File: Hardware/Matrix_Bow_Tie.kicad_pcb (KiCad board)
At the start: 2 copper layers, 17.8 x 13 mm, 9 parts, among them U1 MAX4466

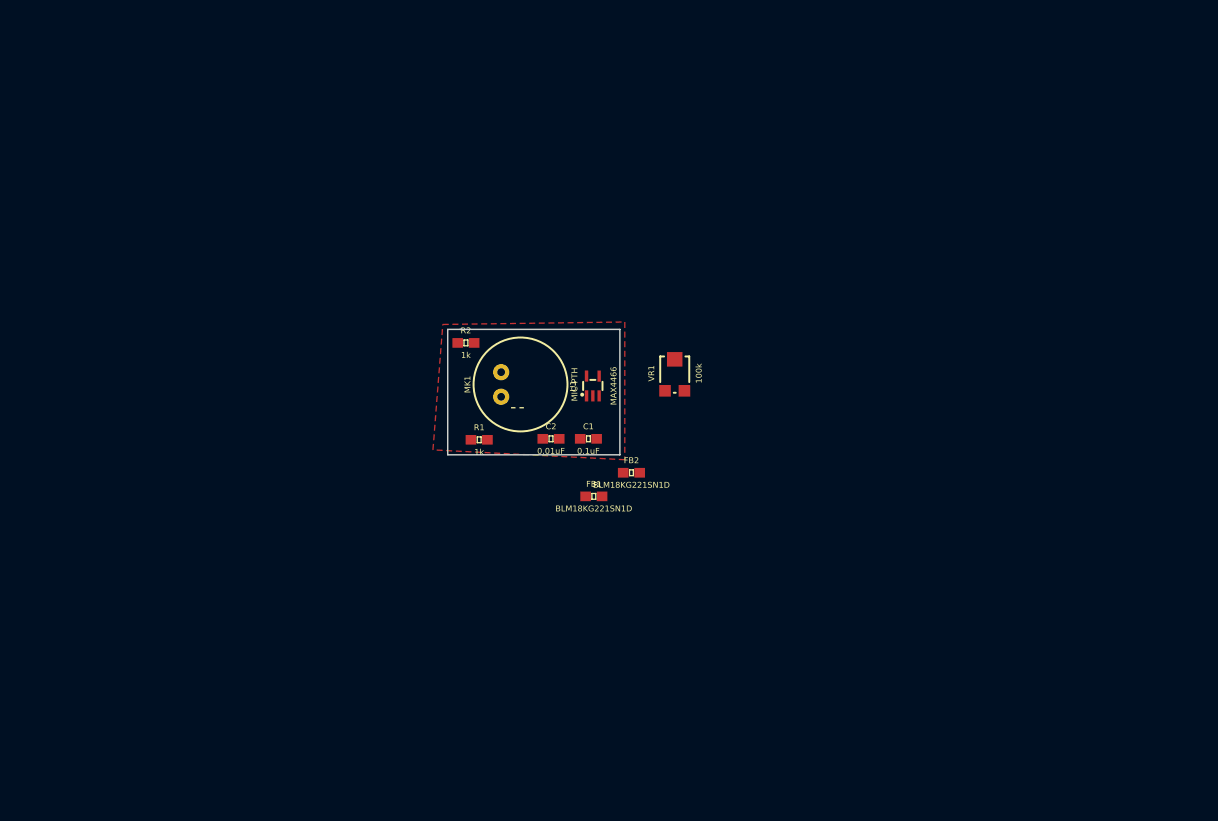
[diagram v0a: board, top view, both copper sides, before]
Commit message: Parts mostly laid out
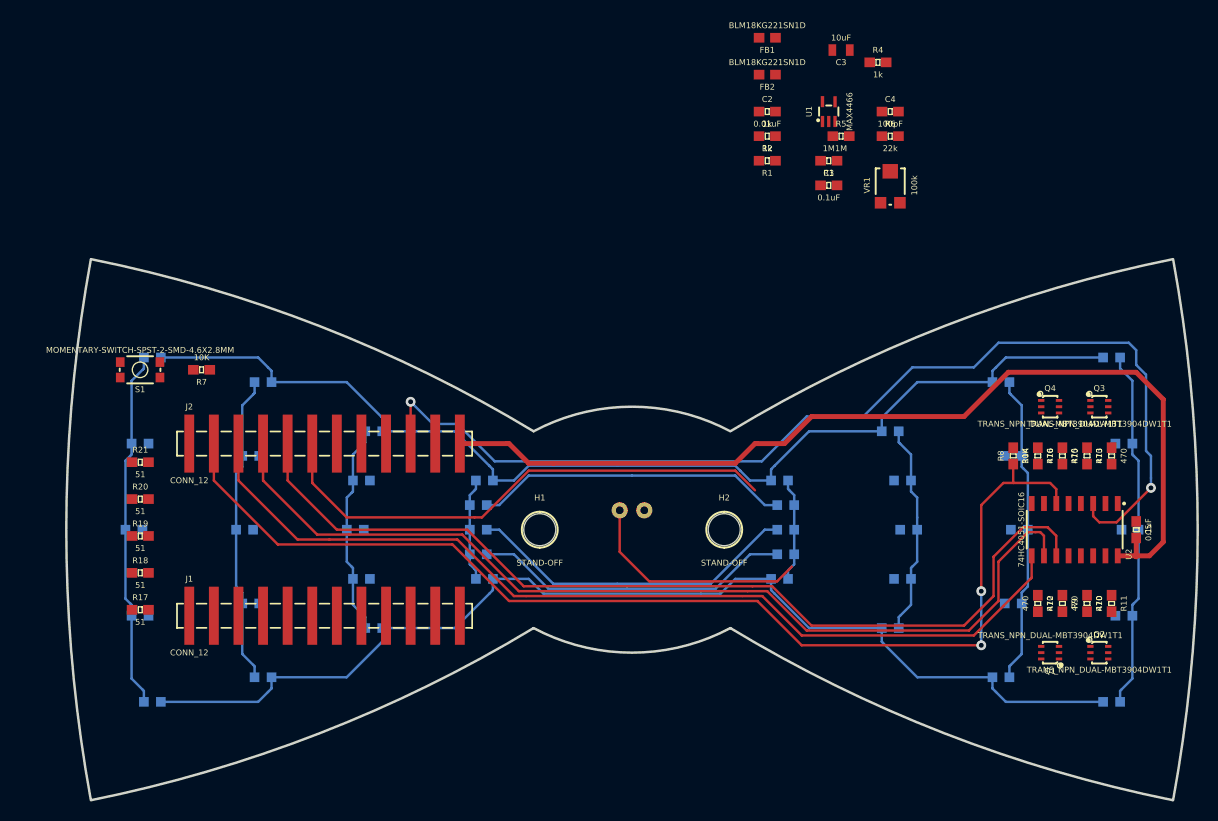
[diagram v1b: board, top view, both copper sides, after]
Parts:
- added C3: 10uF, Capacitors:0805, F.Cu at (181.6, 70.5)
- added C4: 100pF, Capacitors:0603, F.Cu at (186.7, 76.8)
- added C5: 0.1uF, Capacitors:0603, F.Cu at (212.1, 120.0)
- added D1: Yellow, LED:LED-0603, B.Cu at (209.5, 102.2)
- added D10: Yellow, LED:LED-0603, B.Cu at (198.1, 135.2)
- added D11: Yellow, LED:LED-0603, B.Cu at (186.7, 109.8)
- added D12: Yellow, LED:LED-0603, B.Cu at (187.9, 114.9)
- added D13: Yellow, LED:LED-0603, B.Cu at (188.6, 120.0)
- added D14: Yellow, LED:LED-0603, B.Cu at (187.9, 125.1)
- added D15: Yellow, LED:LED-0603, B.Cu at (186.7, 130.2)
- added D16: Yellow, LED:LED-0603, B.Cu at (175.2, 114.9)
- added D17: Yellow, LED:LED-0603, B.Cu at (175.9, 117.5)
- added D18: Yellow, LED:LED-0603, B.Cu at (175.9, 120.0)
- added D19: Yellow, LED:LED-0603, B.Cu at (175.9, 122.5)
- added D2: Yellow, LED:LED-0603, B.Cu at (210.8, 111.1)
- added D20: Yellow, LED:LED-0603, B.Cu at (175.2, 125.1)
- added D21: Yellow, LED:LED-0603, B.Cu at (144.8, 114.9)
- added D22: Yellow, LED:LED-0603, B.Cu at (144.1, 117.5)
- added D23: Yellow, LED:LED-0603, B.Cu at (144.1, 120.0)
- added D24: Yellow, LED:LED-0603, B.Cu at (144.1, 122.5)
- added D25: Yellow, LED:LED-0603, B.Cu at (144.8, 125.1)
- added D26: Yellow, LED:LED-0603, B.Cu at (133.3, 109.8)
- added D27: Yellow, LED:LED-0603, B.Cu at (132.1, 114.9)
- added D28: Yellow, LED:LED-0603, B.Cu at (131.4, 120.0)
- added D29: Yellow, LED:LED-0603, B.Cu at (132.1, 125.1)
- added D3: Yellow, LED:LED-0603, B.Cu at (211.4, 120.0)
- added D30: Yellow, LED:LED-0603, B.Cu at (133.3, 130.2)
- added D31: Yellow, LED:LED-0603, B.Cu at (121.9, 104.8)
- added D32: Yellow, LED:LED-0603, B.Cu at (120.6, 112.4)
- added D33: Yellow, LED:LED-0603, B.Cu at (120.0, 120.0)
- added D34: Yellow, LED:LED-0603, B.Cu at (120.6, 127.6)
- added D35: Yellow, LED:LED-0603, B.Cu at (121.9, 135.2)
- added D36: Yellow, LED:LED-0603, B.Cu at (110.5, 102.2)
- added D37: Yellow, LED:LED-0603, B.Cu at (109.2, 111.1)
- added D38: Yellow, LED:LED-0603, B.Cu at (108.6, 120.0)
- added D39: Yellow, LED:LED-0603, B.Cu at (109.2, 128.9)
- added D4: Yellow, LED:LED-0603, B.Cu at (210.8, 128.9)
- added D40: Yellow, LED:LED-0603, B.Cu at (110.5, 137.8)
- added D5: Yellow, LED:LED-0603, B.Cu at (209.5, 137.8)
- added D6: Yellow, LED:LED-0603, B.Cu at (198.1, 104.8)
- added D7: Yellow, LED:LED-0603, B.Cu at (199.4, 112.4)
- added D8: Yellow, LED:LED-0603, B.Cu at (200.0, 120.0)
- added D9: Yellow, LED:LED-0603, B.Cu at (199.4, 127.6)
- added H1: STAND-OFF, STAND-OFF, F.Cu at (150.5, 120.0)
- added H2: STAND-OFF, STAND-OFF, F.Cu at (169.5, 120.0)
- added J1: CONN_12, Matrix_Bot_Tie:1X12_SMD_MALE, F.Cu at (114.3, 128.9)
- added J2: CONN_12, Matrix_Bot_Tie:1X12_SMD_MALE, F.Cu at (114.3, 111.1)
- added Q1: TRANS_NPN_DUAL-MBT3904DW1T1, Silicon-Standard:SC70-6, F.Cu at (203.2, 132.7)
- added Q2: TRANS_NPN_DUAL-MBT3904DW1T1, Silicon-Standard:SC70-6, F.Cu at (208.3, 132.7)
- added Q3: TRANS_NPN_DUAL-MBT3904DW1T1, Silicon-Standard:SC70-6, F.Cu at (208.3, 107.3)
- added Q4: TRANS_NPN_DUAL-MBT3904DW1T1, Silicon-Standard:SC70-6, F.Cu at (203.2, 107.3)
- added R10: 470, Resistors:0603, F.Cu at (207.0, 127.6)
- added R11: 470, Resistors:0603, F.Cu at (209.5, 127.6)
- added R12: 470, Resistors:0603, F.Cu at (201.9, 127.6)
- added R13: 470, Resistors:0603, F.Cu at (209.5, 112.4)
- added R14: 470, Resistors:0603, F.Cu at (201.9, 112.4)
- added R15: 470, Resistors:0603, F.Cu at (207.0, 112.4)
- added R16: 470, Resistors:0603, F.Cu at (204.4, 112.4)
- added R17: 51, Resistors:0603, F.Cu at (109.2, 128.3)
- added R18: 51, Resistors:0603, F.Cu at (109.2, 124.5)
- added R19: 51, Resistors:0603, F.Cu at (109.2, 120.7)
- added R20: 51, Resistors:0603, F.Cu at (109.2, 116.8)
- added R21: 51, Resistors:0603, F.Cu at (109.2, 113.0)
- added R3: 1M, Resistors:0603, F.Cu at (180.3, 81.9)
- added R4: 1k, Resistors:0603, F.Cu at (185.4, 71.7)
- added R5: 1M, Resistors:0603, F.Cu at (181.6, 79.4)
- added R6: 22k, Resistors:0603, F.Cu at (186.7, 79.4)
- added R7: 10K, Resistors:0603, F.Cu at (115.5, 103.5)
- added R8: 10K, Resistors:0603, F.Cu at (199.4, 112.4)
- added R9: 470, Resistors:0603, F.Cu at (204.4, 127.6)
- added S1: MOMENTARY-SWITCH-SPST-2-SMD-4.6X2.8MM, Switches:TACTILE_SWITCH_SMD_4.6X2.8MM, F.Cu at (109.2, 103.5)
- added U2: 74HC4051-SOIC16, Matrix_Bot_Tie:SOIC-16, F.Cu at (205.7, 120.0)
- C1, C2: footprint 0603 -> Capacitors:0603
- FB1, FB2: footprint 0603 -> Coils:0603
- MK1: footprint MICROPHONE-PTH-9.7MM -> Silicon-Custom:MICROPHONE-PTH-9.7MM; moved to B.Cu
- R1, R2: footprint 0603 -> Resistors:0603
- VR1: footprint TC33X -> Matrix_Bot_Tie:TC33X
- moved FB1 50.6 mm to (174.0, 69.2), turned to 180 degrees
- moved FB2 43.4 mm to (174.0, 73.0), turned to 180 degrees
- moved R1 41.4 mm to (174.0, 81.9), turned to 180 degrees
- moved C2 40.5 mm to (174.0, 76.8)
- moved R2 37.7 mm to (174.0, 79.4), turned to 180 degrees
- moved U1 37.4 mm to (180.3, 76.8)
- moved C1 36.1 mm to (180.3, 84.4)
- moved VR1 29.5 mm to (186.7, 84.4)
- moved MK1 18.9 mm to (160.0, 120.0), turned to 270 degrees
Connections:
- U1 pad 1: Net-(U1-Pad1) -> Net-(C2-Pad2)
- U1 pad 4: Net-(U1-Pad4) -> OUT
- U1 pad 5: Net-(U1-Pad5) -> VCCA
- VR1 pad 1: Net-(U1-Pad4) -> OUT
- VR1 pad 2: Net-(VR1-Pad2) -> OUT
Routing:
- net E: track 0.00 -> 117.0 mm, vias 0 -> 2
- net Net-(D10-PadA): track 0.00 -> 113.5 mm
- net Net-(D1-PadA): track 0.00 -> 113.5 mm
- net Z: track 0.00 -> 111.0 mm, vias 0 -> 2
- net 3.3V: track 0.00 -> 100.6 mm
- net S1: track 0.00 -> 99.7 mm
- net S0: track 0.00 -> 98.4 mm
- net S2: track 0.00 -> 97.1 mm
- net OUT: track 0.00 -> 54.1 mm
- net Net-(D36-PadC): track 0.00 -> 37.1 mm
- net Net-(D1-PadC): track 0.00 -> 37.1 mm
- net Net-(D13-PadA): track 0.00 -> 34.6 mm
- net Net-(D14-PadA): track 0.00 -> 32.9 mm
- net Net-(D12-PadA): track 0.00 -> 32.5 mm
- net Net-(D31-PadC): track 0.00 -> 32.1 mm
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- removed copper zone on F.Cu, net AGND
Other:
- board size 17.8 x 13 mm -> 116.8 x 55.9 mm
- net class Default: clearance 0.254 -> 0.2032; via_dia 0.6 -> 1.016; via_drill 0.4 -> 0.508
- net class Power added: clearance 0.2032, trace_width 0.508, via_dia 1.016, via_drill 0.508
- rule trace_clearance: 0.254 -> 0.2032
